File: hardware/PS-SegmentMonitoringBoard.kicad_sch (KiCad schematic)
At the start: 3 parts, among them J4 24V_Conn

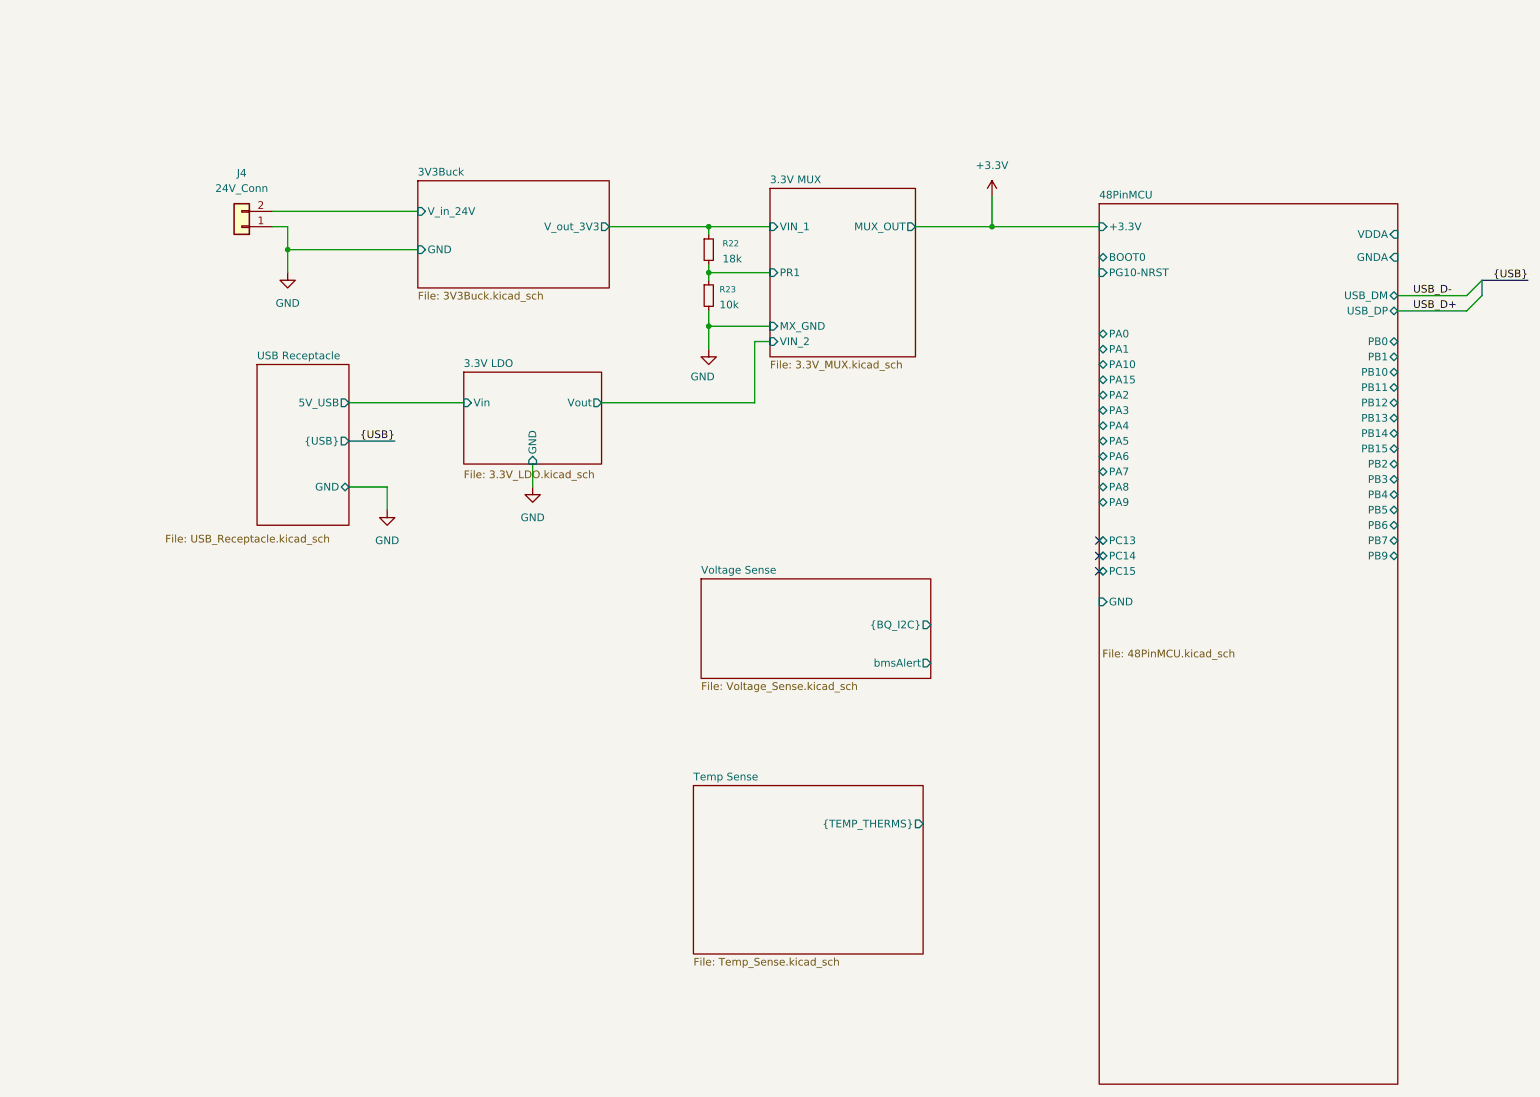
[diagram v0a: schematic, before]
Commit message: schem except BQ
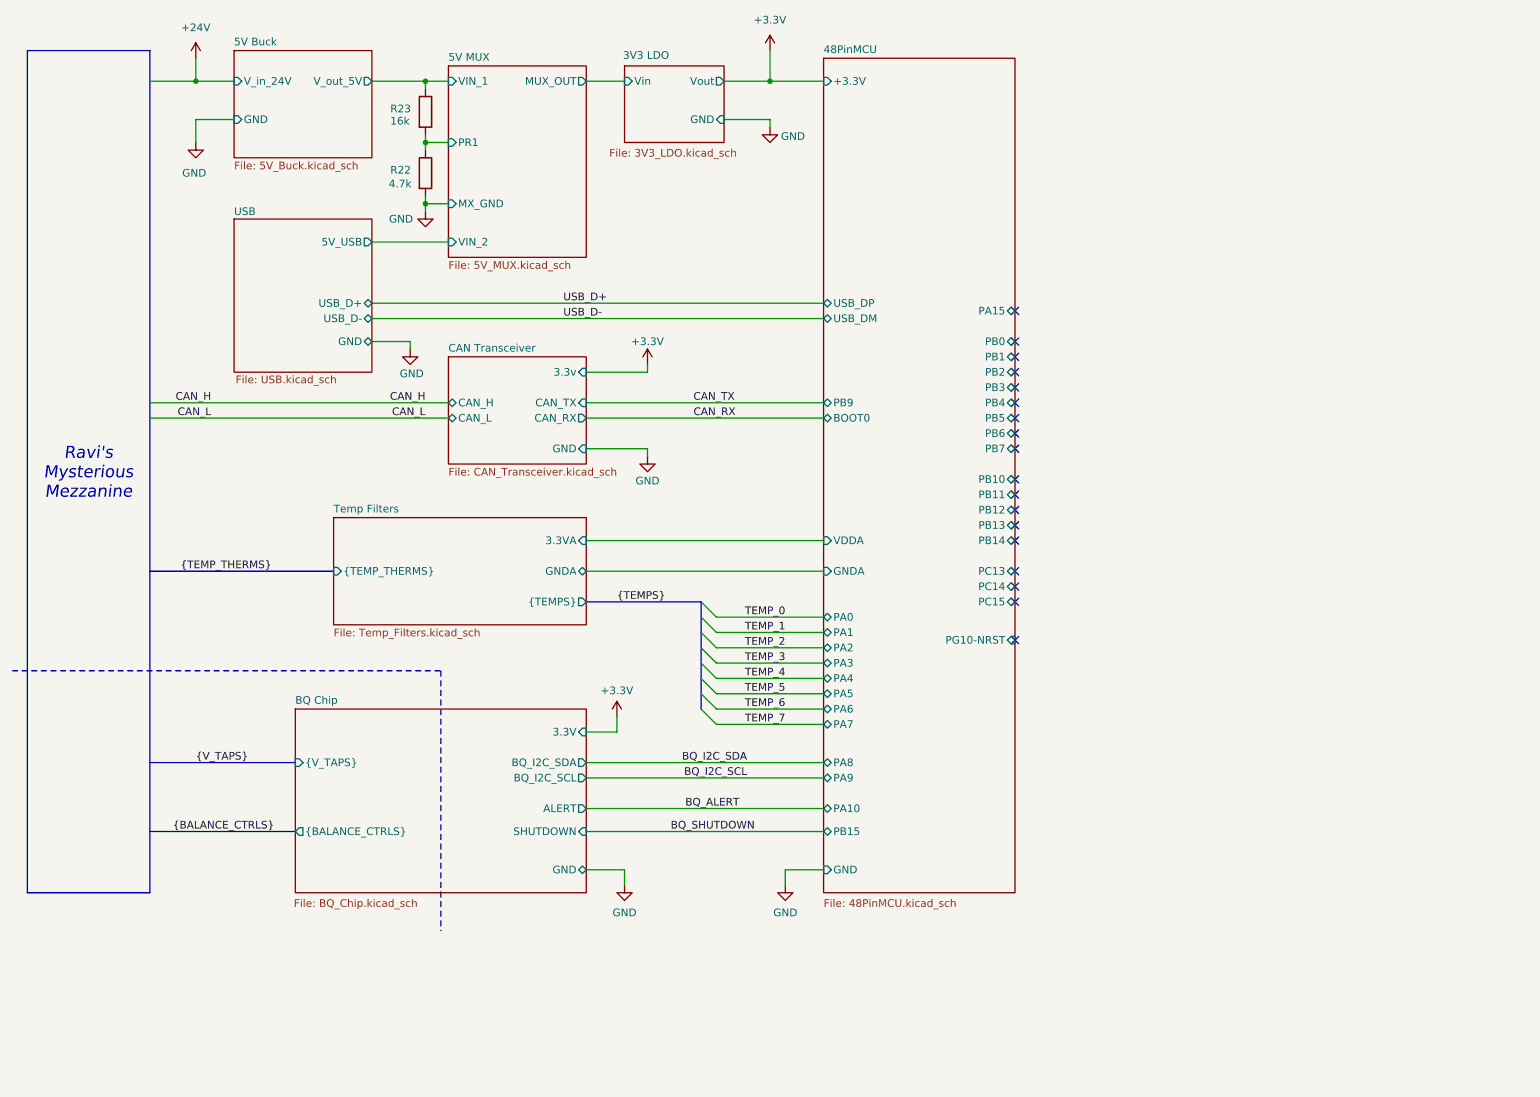
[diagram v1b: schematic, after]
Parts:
- removed J4: 24V_Conn, symbol Connector_Generic:Conn_01x02
- removed R22: 18k, symbol Device:R_Small
- removed R23: 10k, symbol Device:R_Small
- added R22: 4.7k, symbol Device:R
- added R23: 16k, symbol Device:R
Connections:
- net GND: now also R22.2
- new net 5V Buck/V_out_5V: R23.1
- new net 5V MUX/PR1: R22.1, R23.2
- no-connect marks 3 -> 18
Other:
- sheet 3V3Buck renamed 5V Buck
- sheet USB Receptacle renamed USB
- sheet Voltage Sense renamed BQ Chip
- removed sheet 3.3V LDO
- removed sheet 3.3V MUX
- removed sheet Temp Sense
- added sheet 3V3 LDO (3V3_LDO.kicad_sch)
- added sheet 5V MUX (5V_MUX.kicad_sch)
- added sheet CAN Transceiver (CAN_Transceiver.kicad_sch)
- added sheet Temp Filters (Temp_Filters.kicad_sch)
- sheet 5V Buck: file 3V3Buck.kicad_sch -> 5V_Buck.kicad_sch
- sheet 5V Buck ports: added V_out_5V; removed V_out_3V3
- sheet BQ Chip: file Voltage_Sense.kicad_sch -> BQ_Chip.kicad_sch
- sheet BQ Chip ports: added 3.3V, ALERT, BQ_I2C_SCL, BQ_I2C_SDA, GND, SHUTDOWN, {BALANCE_CTRLS}, {V_TAPS}; removed bmsAlert, {BQ_I2C}
- sheet USB: file USB_Receptacle.kicad_sch -> USB.kicad_sch
- sheet USB ports: added USB_D+, USB_D-; removed {USB}
- note added: "Ravi's Mysterious Mezzanine"
